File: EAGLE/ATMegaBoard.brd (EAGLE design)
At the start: 91.4 x 69.5 mm, 29 parts, among them IC1 L298, IC2 ATMEGA168-20P, IC3 REG1117, J1 1X2-3.5MM, J2 1X2-3.5MM, J3 1X2-3.5MM, J4 1X2-3.5MM, X1 49S/18PF

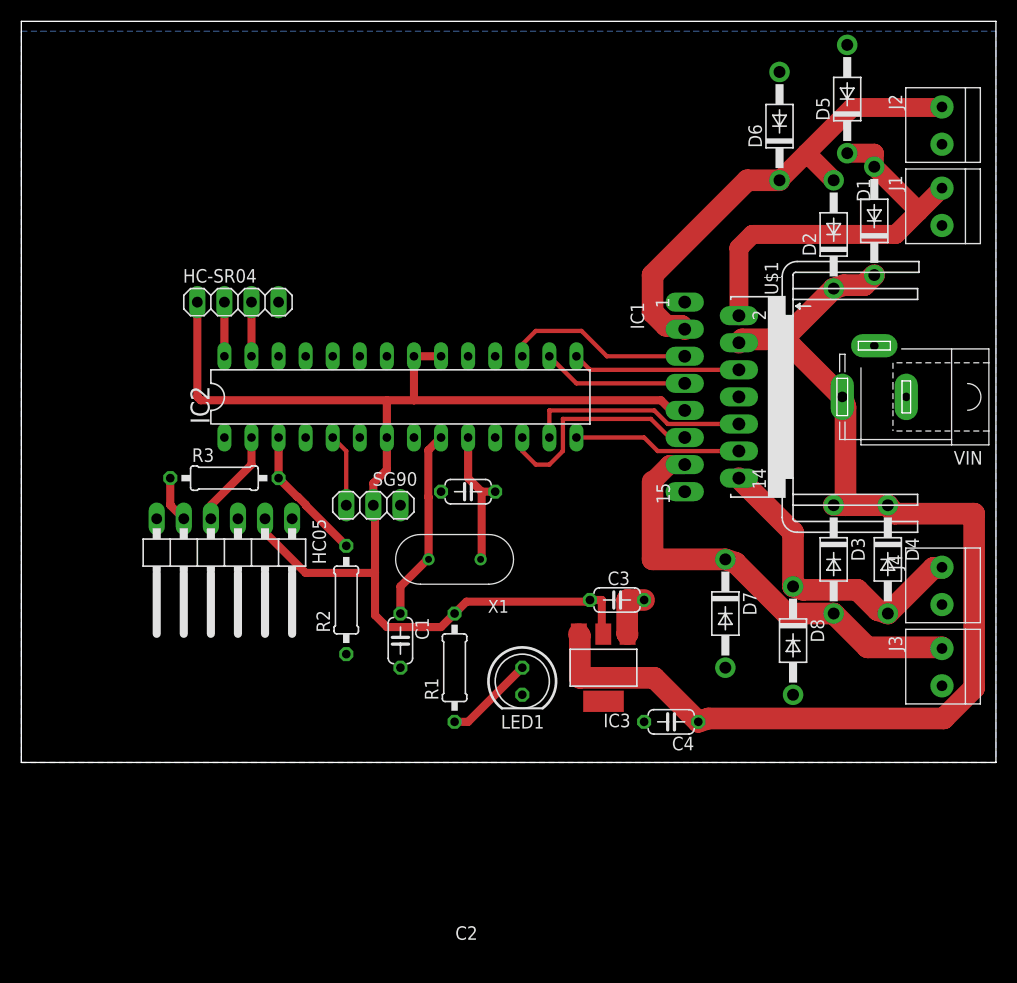
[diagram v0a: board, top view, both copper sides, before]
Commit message: added standalone board
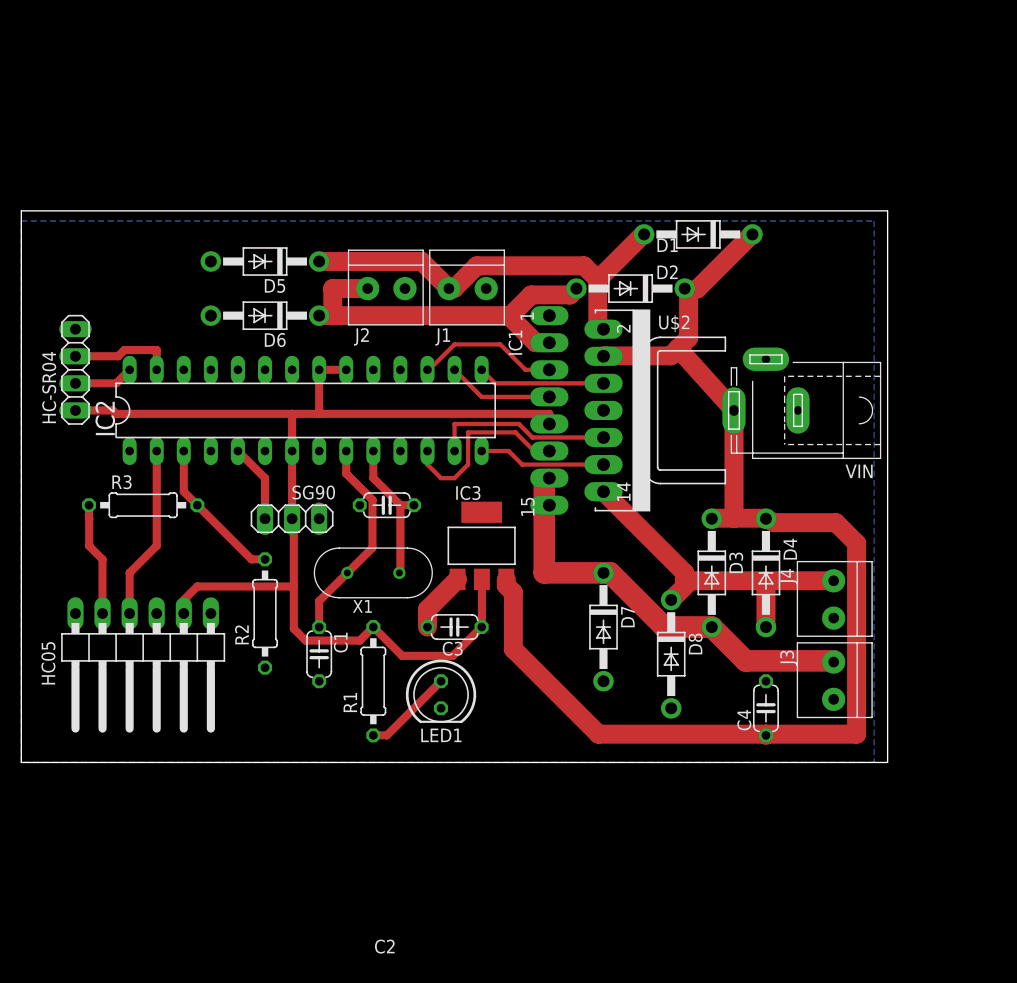
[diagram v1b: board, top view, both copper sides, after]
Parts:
- removed U$1: (no value), heatsink:FK213
- added U$2: (no value), heatsink:D03S
- moved D5 56.7 mm to (22.9, 47.0), turned to 180 degrees
- moved J2 54.3 mm to (34.3, 44.5), turned to 180 degrees
- moved D6 51.4 mm to (22.9, 41.9), turned to 180 degrees
- moved J1 45.1 mm to (41.9, 44.5), turned to 180 degrees
- moved D2 19.7 mm to (57.1, 44.5), turned to 180 degrees
- moved D1 16.6 mm to (63.5, 49.5), turned to 180 degrees
- moved HC-SR04 16.5 mm to (5.08, 36.8), turned to 90 degrees
- moved IC3 16.2 mm to (43.2, 20.3), turned to 0 degrees
- moved C3 15.5 mm to (40.6, 12.7), turned to 180 degrees
- moved IC1 12.8 mm to (57.1, 33.0)
- moved HC05 11.7 mm to (11.4, 10.2)
- moved D3 11.5 mm to (64.8, 17.8)
- moved D4 11.5 mm to (69.8, 17.8)
- moved D7 11.5 mm to (54.6, 12.7)
- moved D8 11.5 mm to (61.0, 10.2)
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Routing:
- net +5V: track 121.8 -> 109.8 mm
- net OUT2: track 44.5 -> 35.9 mm
- net VIN: track 107.2 -> 114.4 mm
- net TX: track 9.20 -> 16.3 mm
- net PIN5HC05: track 4.34 -> 10.7 mm
- net ECHO: track 5.08 -> 9.72 mm
- net IN1: track 17.9 -> 13.4 mm
- net IN3: track 20.8 -> 17.0 mm
- net ENA: track 15.8 -> 12.0 mm
- net IN4: track 15.8 -> 12.0 mm
- net IN2: track 13.8 -> 9.94 mm
- net ENB: track 21.3 -> 17.5 mm
- net OUT4: track 29.0 -> 32.4 mm
- net OUT1: track 37.4 -> 39.6 mm
- net OUT3: track 41.6 -> 39.9 mm
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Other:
- board size 91.4 x 69.5 mm -> 81.3 x 51.7 mm
